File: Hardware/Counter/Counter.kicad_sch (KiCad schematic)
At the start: 25 parts, among them J1 PWR, J2 OUT, SW1 SW_Push, SW2 SW_Push, SW3 SW_Push, U1 LM555xM

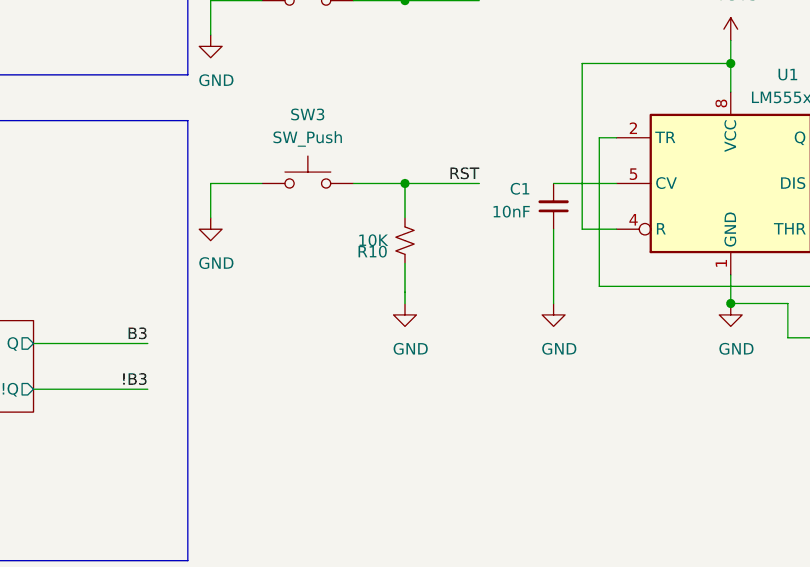
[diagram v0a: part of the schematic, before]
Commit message: kicad updates
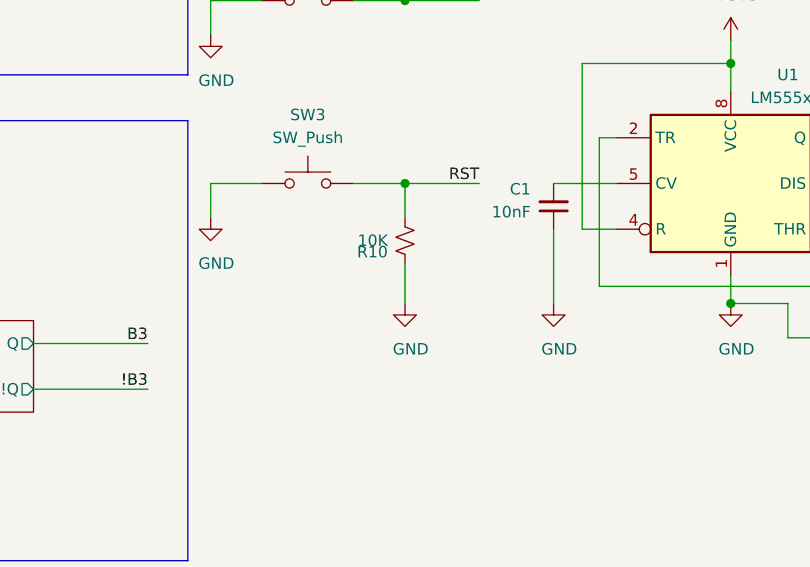
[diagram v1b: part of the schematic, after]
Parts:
- J1: Spice_Model (none) -> dc 3.3; Spice_Netlist_Enabled (none) -> Y; Spice_Primitive (none) -> I
- SW1: Spice_Model (none) -> ac 3.3 pulse(0 3.3 1n 1n 1n 1n 2n); Spice_Netlist_Enabled (none) -> Y; Spice_Primitive (none) -> I
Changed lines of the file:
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@@
     (stroke (width 0) (type solid) (color 0 0 0 0))
   )
-  (wire (pts (xy 180.34 156.845) (xy 180.34 153.67))
-    (stroke (width 0) (type solid) (color 0 0 0 0))
-  )
-  (wire (pts (xy 180.34 156.845) (xy 180.34 158.115))
+  (wire (pts (xy 180.34 153.67) (xy 180.34 158.115))
     (stroke (width 0) (type solid) (color 0 0 0 0))
   )
@@
       (effects (font (size 1.27 1.27)) hide)
     )
+    (property "Spice_Primitive" "I" (id 4) (at 271.78 128.905 0)
+      (effects (font (size 1.27 1.27)) hide)
+    )
+    (property "Spice_Model" "dc 3.3" (id 5) (at 271.78 128.905 0)
+      (effects (font (size 1.27 1.27)) hide)
+    )
+    (property "Spice_Netlist_Enabled" "Y" (id 6) (at 271.78 128.905 0)
+      (effects (font (size 1.27 1.27)) hide)
+    )
   )
   (symbol (lib_id "Switch:SW_Push") (at 169.545 101.6 0) (unit 1)
@@
       (effects (font (size 1.27 1.27)) hide)
     )
+    (property "Spice_Primitive" "I" (id 4) (at 169.545 101.6 0)
+      (effects (font (size 1.27 1.27)) hide)
+    )
+    (property "Spice_Model" "ac 3.3 pulse(0 3.3 1n 1n 1n 1n 2n)" (id 5) (at 169.545 101.6 0)
+      (effects (font (size 1.27 1.27)) hide)
+    )
+    (property "Spice_Netlist_Enabled" "Y" (id 6) (at 169.545 101.6 0)
+      (effects (font (size 1.27 1.27)) hide)
+    )
